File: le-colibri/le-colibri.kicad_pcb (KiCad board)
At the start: 2 copper layers, 225.8 x 89.3 mm, 63 parts, among them SW1 CPG151101S11, SW10 CPG151101S11, SW11 CPG151101S11, SW12 CPG151101S11, SW13 CPG151101S11, SW14 CPG151101S11, SW15 CPG151101S11, SW16 CPG151101S11, SW17 CPG151101S11, SW18 CPG151101S11, SW19 CPG151101S11, SW2 CPG151101S11, SW20 CPG151101S11, SW21 CPG151101S11, SW22 CPG151101S11, SW23 CPG151101S11, SW24 CPG151101S11, SW25 CPG151101S11, SW26 CPG151101S11, SW27 CPG151101S11, SW28 CPG151101S11, SW29 CPG151101S11, SW3 CPG151101S11, SW30 CPG151101S11, SW4 CPG151101S11, SW5 CPG151101S11, SW6 CPG151101S11, SW7 CPG151101S11, SW8 CPG151101S11, SW9 CPG151101S11, U1 Seeeduino Xiao rp2040

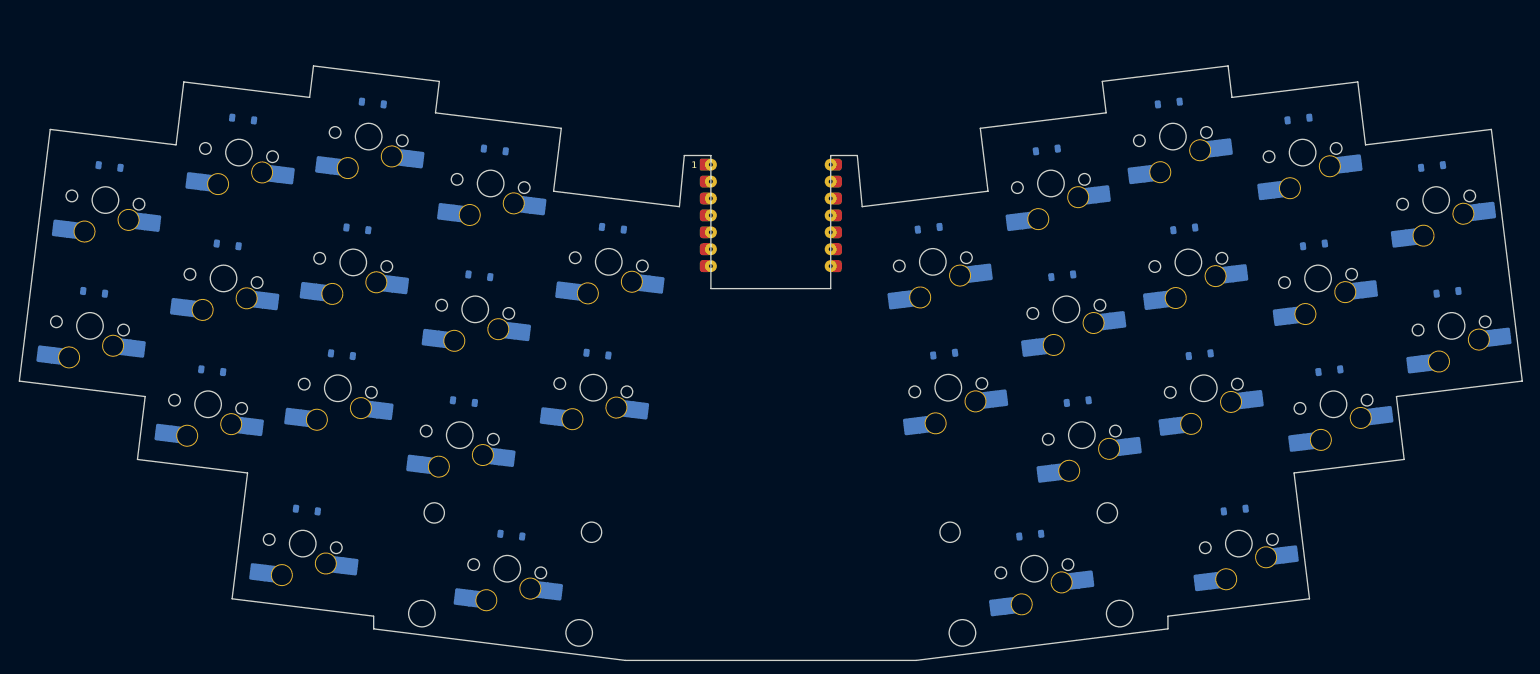
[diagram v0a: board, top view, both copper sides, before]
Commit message: "first" "release"
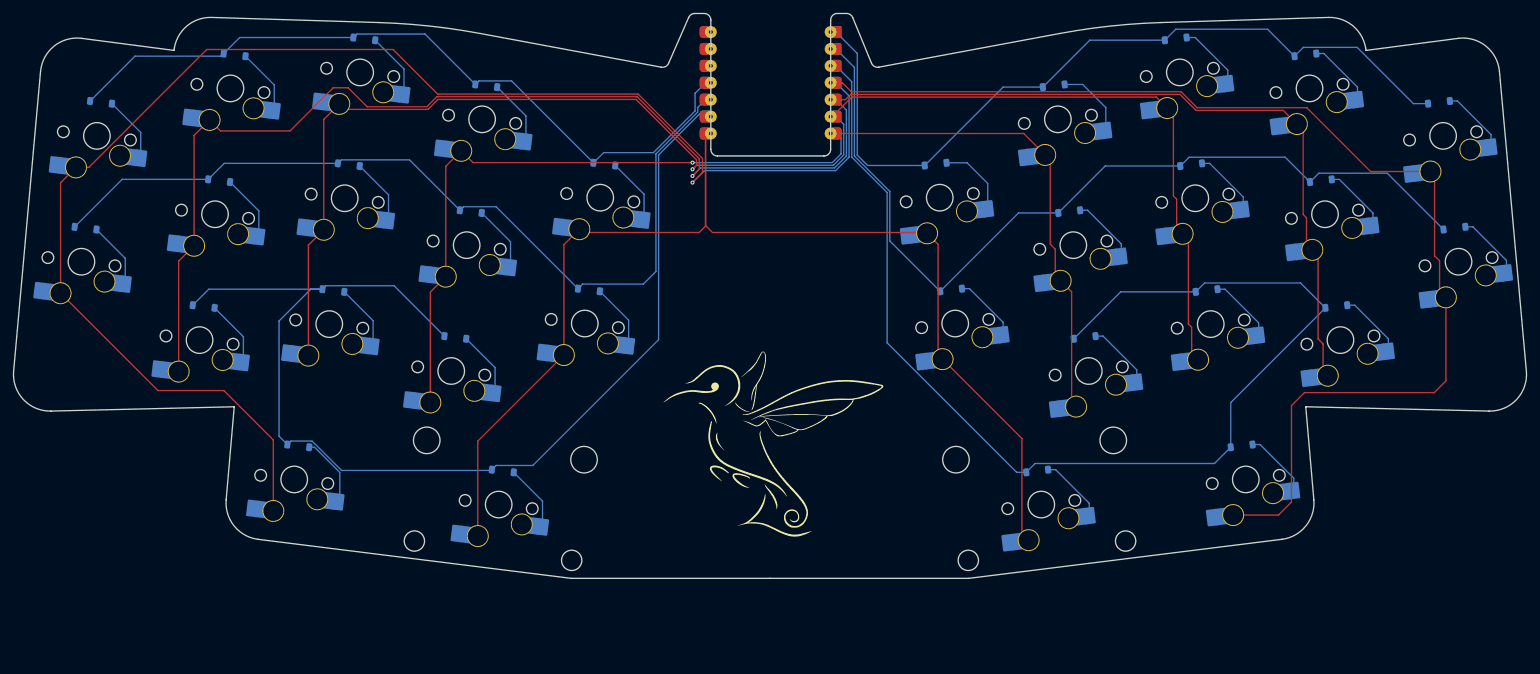
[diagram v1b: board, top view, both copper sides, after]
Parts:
- added G***: LOGO, LOGO, F.Cu at (151.0, 106.1)
- added G***: LOGO, LOGO, B.Cu at (151.0, 106.1)
- U1: moved to B.Cu
- moved U1 19.9 mm to (150.9, 52.6), turned to 180 degrees
- moved D12 9.73 mm to (85.2, 83.8)
- moved D15 9.73 mm to (110.7, 110.9)
- moved D5 9.73 mm to (125.9, 64.8)
- moved D6 9.73 mm to (48.0, 74.4)
- moved D9 9.73 mm to (105.8, 71.9)
- moved SW1 9.73 mm to (49.7, 60.6)
- moved SW11 9.73 mm to (65.1, 91.3)
- moved SW12 9.73 mm to (84.6, 88.9)
- moved SW14 9.73 mm to (79.3, 112.2)
- moved SW8 9.73 mm to (86.9, 69.9)
- moved SW9 9.73 mm to (105.2, 77.0)
- moved D3 9.73 mm to (89.8, 46.0)
- moved SW3 9.73 mm to (89.2, 51.0)
- moved SW4 9.73 mm to (107.6, 58.1)
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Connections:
- U1 pad 1: unconnected-(U1-P26-Pad1) -> R4
- U1 pad 11: unconnected-(U1-P3-Pad11) -> R1
- U1 pad 12: unconnected-(U1-P4-Pad12) -> R2
- U1 pad 13: unconnected-(U1-P2-Pad13) -> R3
- U1 pad 14: unconnected-(U1-P1-Pad14) -> C5
- U1 pad 2: unconnected-(U1-P27-Pad2) -> R5
- U1 pad 3: unconnected-(U1-P28-Pad3) -> R6
- U1 pad 4: unconnected-(U1-P29-Pad4) -> C1
- U1 pad 5: unconnected-(U1-P6-Pad5) -> C2
- U1 pad 6: unconnected-(U1-P7-Pad6) -> C3
- U1 pad 7: unconnected-(U1-P0-Pad7) -> C4
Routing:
- net C1: track 0.00 -> 397.3 mm, vias 0 -> 1
- net C2: track 0.00 -> 270.0 mm, vias 0 -> 1
- net C3: track 0.00 -> 221.4 mm, vias 0 -> 1
- net C5: track 0.00 -> 186.0 mm
- net R6: track 0.00 -> 175.7 mm
- net C4: track 0.00 -> 174.0 mm, vias 0 -> 1
- net R3: track 0.00 -> 173.4 mm
- net R5: track 0.00 -> 132.5 mm
- net R2: track 0.00 -> 129.9 mm
- net R4: track 0.00 -> 120.5 mm
- net R1: track 0.00 -> 111.6 mm
- net Net-(D16-K): track 0.00 -> 11.3 mm
- net Net-(D17-K): track 0.00 -> 11.1 mm
- net Net-(D14-K): track 0.00 -> 10.7 mm
- net Net-(D18-K): track 0.00 -> 10.2 mm
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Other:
- board size 225.8 x 89.3 mm -> 227.4 x 84.9 mm
- board text added: "Le Colibri"
- board text added: "© 2024 Travis Mick github.com/eggsworks"
